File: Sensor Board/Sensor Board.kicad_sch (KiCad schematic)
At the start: 32 parts, among them J1 Programming Header, J3 Micro_SD_Card, U1 PIC18F26K83, U2 SPX3819M5-L-3-3, U3 MCP2562, Y1 12MHz Crystal

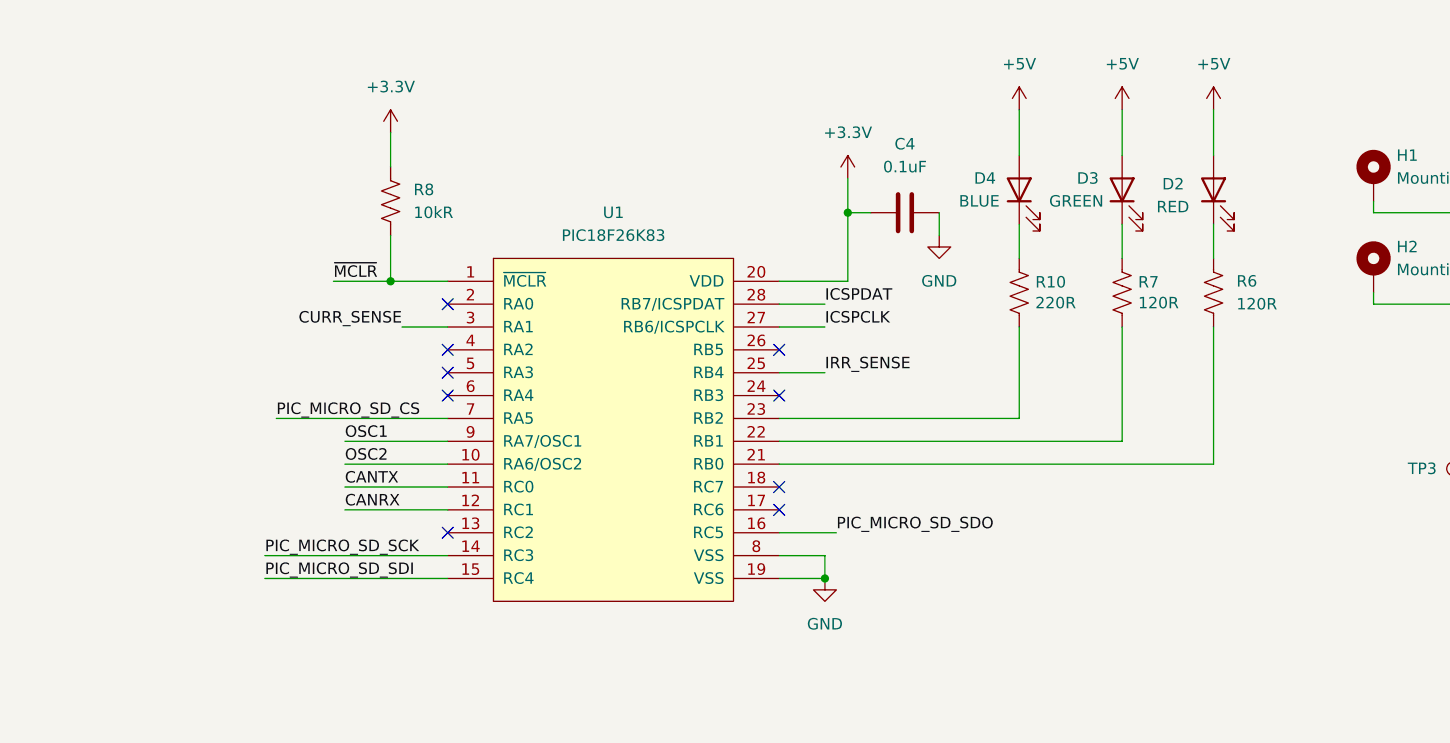
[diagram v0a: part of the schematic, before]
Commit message: Cooked another layout-Pranav
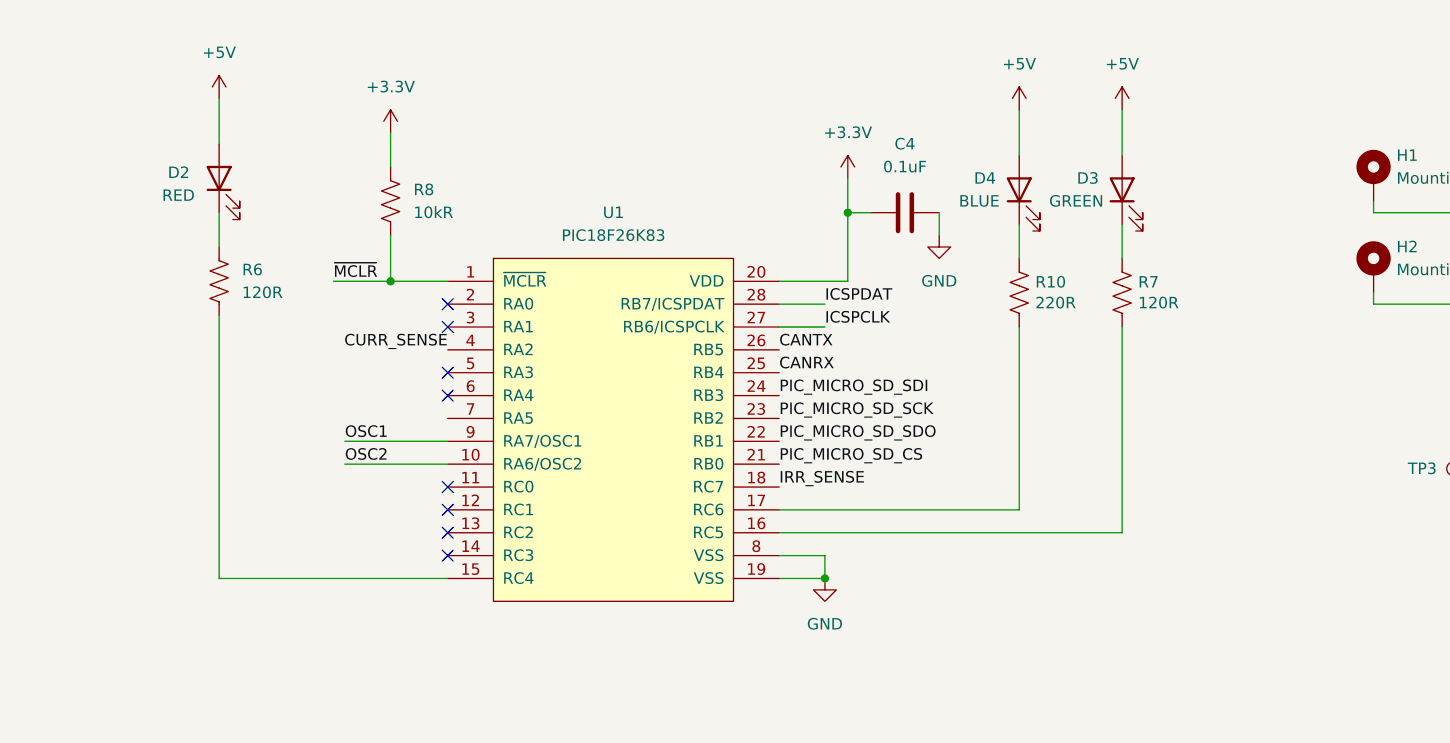
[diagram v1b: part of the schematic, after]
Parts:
- Y1: value 12MHz Crystal -> 12MHz Crystal
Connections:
- net CANRX: now also U1.25 (RB4); no longer U1.12 (RC1)
- net CANTX: now also U1.26 (RB5); no longer U1.11 (RC0)
- net CURR_SENSE: now also U1.4 (RA2); no longer U1.3 (RA1)
- net IRR_SENSE: now also U1.18 (RC7); no longer U1.25 (RB4)
- net PIC_MICRO_SD_CS: now also U1.21 (RB0); no longer U1.7 (RA5)
- net PIC_MICRO_SD_SCK: now also U1.23 (RB2); no longer U1.14 (RC3)
- net PIC_MICRO_SD_SDI: now also U1.24 (RB3); no longer U1.15 (RC4)
- net PIC_MICRO_SD_SDO: now also U1.22 (RB1); no longer U1.16 (RC5)
- net at U1.17 (RC6): now also R10.2
- net at R6.2: now also U1.15 (RC4); no longer U1.21 (RB0)
- net at R7.2: now also U1.16 (RC5); no longer U1.22 (RB1)
- no-connect marks 9 -> 8
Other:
- moved on the sheet: D2, R6
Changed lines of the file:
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@@
 	)
 	(no_connect
-		(at 162.56 73.66)
+		(at 125.73 78.74)
 	)
 	(no_connect
-		(at 125.73 60.96)
+		(at 125.73 53.34)
 	)
 	(no_connect
-		(at 162.56 71.12)
+		(at 125.73 60.96)
 	)
 	(no_connect
-		(at 125.73 50.8)
+		(at 125.73 73.66)
 	)
 	(no_connect
@@
 	)
 	(no_connect
-		(at 162.56 60.96)
-	)
-	(no_connect
-		(at 162.56 55.88)
+		(at 125.73 50.8)
 	)
 	(no_connect
@@
 	)
 	(no_connect
-		(at 125.73 55.88)
+		(at 125.73 71.12)
 	)
 	(wire
@@
 	(wire
 		(pts
-			(xy 200.66 29.21) (xy 200.66 34.29)
+			(xy 100.33 81.28) (xy 125.73 81.28)
 		)
 		(stroke
@@
 	(wire
 		(pts
-			(xy 120.65 53.34) (xy 125.73 53.34)
+			(xy 200.66 29.21) (xy 200.66 34.29)
 		)
 		(stroke
@@
 	(wire
 		(pts
-			(xy 210.82 29.21) (xy 210.82 34.29)
-		)
-		(stroke
-			(width 0)
-			(type default)
-		)
-	)
-	(wire
-		(pts
-			(xy 210.82 53.34) (xy 210.82 68.58)
+			(xy 100.33 27.94) (xy 100.33 33.02)
 		)
 		(stroke
@@
 	(wire
 		(pts
-			(xy 210.82 41.91) (xy 210.82 45.72)
+			(xy 100.33 40.64) (xy 100.33 44.45)
 		)
 		(stroke
@@
 	(wire
 		(pts
-			(xy 189.23 41.91) (xy 189.23 45.72)
+			(xy 200.66 53.34) (xy 200.66 76.2)
 		)
 		(stroke
@@
 	(wire
 		(pts
-			(xy 162.56 58.42) (xy 167.64 58.42)
+			(xy 189.23 41.91) (xy 189.23 45.72)
 		)
 		(stroke
@@
 	(wire
 		(pts
-			(xy 114.3 71.12) (xy 125.73 71.12)
-		)
-		(stroke
-			(width 0)
-			(type default)
-		)
-	)
-	(wire
-		(pts
 			(xy 85.09 134.62) (xy 85.09 138.43)
 		)
@@
 	(wire
 		(pts
-			(xy 162.56 66.04) (xy 200.66 66.04)
-		)
-		(stroke
-			(width 0)
-			(type default)
-		)
-	)
-	(wire
-		(pts
 			(xy 261.62 95.25) (xy 261.62 88.9)
 		)
@@
 	(wire
 		(pts
-			(xy 162.56 76.2) (xy 168.91 76.2)
-		)
-		(stroke
-			(width 0)
-			(type default)
-		)
-	)
-	(wire
-		(pts
 			(xy 125.73 115.57) (xy 125.73 113.03)
 		)
@@
 	(wire
 		(pts
-			(xy 105.41 81.28) (xy 125.73 81.28)
+			(xy 170.18 40.64) (xy 170.18 48.26)
 		)
 		(stroke
@@
 	(wire
 		(pts
-			(xy 170.18 40.64) (xy 170.18 48.26)
+			(xy 189.23 29.21) (xy 189.23 34.29)
 		)
 		(stroke
@@
 	(wire
 		(pts
-			(xy 189.23 29.21) (xy 189.23 34.29)
+			(xy 162.56 53.34) (xy 167.64 53.34)
 		)
 		(stroke
@@
 	(wire
 		(pts
-			(xy 162.56 53.34) (xy 167.64 53.34)
+			(xy 248.92 115.57) (xy 251.46 115.57)
 		)
 		(stroke
@@
 	(wire
 		(pts
-			(xy 248.92 115.57) (xy 251.46 115.57)
+			(xy 237.49 72.39) (xy 237.49 77.47)
 		)
 		(stroke
@@
 	(wire
 		(pts
-			(xy 237.49 72.39) (xy 237.49 77.47)
+			(xy 100.33 52.07) (xy 100.33 81.28)
 		)
 		(stroke
@@
 	(wire
 		(pts
-			(xy 200.66 53.34) (xy 200.66 66.04)
+			(xy 162.56 73.66) (xy 189.23 73.66)
 		)
 		(stroke
@@
 	(wire
 		(pts
-			(xy 189.23 53.34) (xy 189.23 63.5)
+			(xy 189.23 53.34) (xy 189.23 73.66)
 		)
 		(stroke
@@
 	(wire
 		(pts
-			(xy 114.3 73.66) (xy 125.73 73.66)
-		)
-		(stroke
-			(width 0)
-			(type default)
-		)
-	)
-	(wire
-		(pts
 			(xy 200.66 45.72) (xy 200.66 41.91)
 		)
@@
 	(wire
 		(pts
-			(xy 105.41 78.74) (xy 125.73 78.74)
-		)
-		(stroke
-			(width 0)
-			(type default)
-		)
-	)
-	(wire
-		(pts
 			(xy 144.78 113.03) (xy 166.37 113.03)
 		)
@@
 	(wire
 		(pts
-			(xy 21.59 119.38) (xy 21.59 123.19)
+			(xy 200.66 76.2) (xy 162.56 76.2)
 		)
 		(stroke
@@
 	(wire
 		(pts
-			(xy 172.72 40.64) (xy 170.18 40.64)
+			(xy 21.59 119.38) (xy 21.59 123.19)
 		)
 		(stroke
@@
 	(wire
 		(pts
-			(xy 106.68 63.5) (xy 125.73 63.5)
+			(xy 172.72 40.64) (xy 170.18 40.64)
 		)
 		(stroke
@@
 	(wire
 		(pts
-			(xy 162.56 68.58) (xy 210.82 68.58)
-		)
-		(stroke
-			(width 0)
-			(type default)
-		)
-	)
-	(wire
-		(pts
 			(xy 114.3 66.04) (xy 125.73 66.04)
 		)
@@
 	(wire
 		(pts
-			(xy 189.23 63.5) (xy 162.56 63.5)
-		)
-		(stroke
-			(width 0)
-			(type default)
-		)
-	)
-	(wire
-		(pts
 			(xy 48.26 181.61) (xy 48.26 161.29)
 		)
@@
 	)
 	(label "IRR_SENSE"
-		(at 167.64 58.42 0)
+		(at 162.56 71.12 0)
 		(fields_autoplaced yes)
 		(effects
@@
 	)
 	(label "CANTX"
-		(at 114.3 71.12 0)
+		(at 162.56 55.88 0)
 		(fields_autoplaced yes)
 		(effects
@@
 	)
 	(label "PIC_MICRO_SD_SCK"
-		(at 105.41 78.74 0)
+		(at 162.56 63.5 0)
 		(fields_autoplaced yes)
 		(effects
@@
 	)
 	(label "CANRX"
-		(at 114.3 73.66 0)
+		(at 162.56 58.42 0)
 		(fields_autoplaced yes)
 		(effects
@@
 	)
 	(label "PIC_MICRO_SD_SDO"
-		(at 168.91 76.2 0)
+		(at 162.56 66.04 0)
 		(fields_autoplaced yes)
 		(effects
@@
 	)
 	(label "PIC_MICRO_SD_SDI"
-		(at 105.41 81.28 0)
+		(at 162.56 60.96 0)
 		(fields_autoplaced yes)
 		(effects
@@
 	)
 	(label "PIC_MICRO_SD_CS"
-		(at 106.68 63.5 0)
+		(at 162.56 68.58 0)
 		(fields_autoplaced yes)
 		(effects
@@
 	)
 	(label "CURR_SENSE"
-		(at 120.65 53.34 180)
+		(at 125.73 55.88 180)
 		(fields_autoplaced yes)
 		(effects
@@
 			)
 		)
-		(property "Value" "12MHz Crystal "
+		(property "Value" "12MHz Crystal"
 			(at 38.8874 111.633 90)
 			(effects
@@
 		(lib_name "+5V_3")
 		(lib_id "power:+5V")
-		(at 210.82 29.21 0)
+		(at 100.33 27.94 0)
 		(unit 1)
 		(exclude_from_sim no)
@@
 		(fields_autoplaced yes)
 		(property "Reference" "#PWR06"
-			(at 210.82 33.02 0)
+			(at 100.33 31.75 0)
 			(effects
 				(font
@@
 		)
 		(property "Value" "+5V"
-			(at 210.82 24.13 0)
+			(at 100.33 22.86 0)
 			(effects
 				(font
@@
 		)
 		(property "Footprint" ""
-			(at 210.82 29.21 0)
+			(at 100.33 27.94 0)
 			(effects
 				(font
@@
 		)
 		(property "Datasheet" ""
-			(at 210.82 29.21 0)
+			(at 100.33 27.94 0)
 			(effects
 				(font
@@
 		)
 		(property "Description" "Power symbol creates a global label with name \"+5V\""
-			(at 210.82 29.21 0)
+			(at 100.33 27.94 0)
 			(effects
 				(font
@@
 	(symbol
 		(lib_id "Device:LED")
-		(at 210.82 38.1 90)
+		(at 100.33 36.83 90)
 		(unit 1)
 		(exclude_from_sim no)
@@
 		(dnp no)
 		(property "Reference" "D2"
-			(at 205.105 37.465 90)
+			(at 94.615 36.195 90)
 			(effects
 				(font
@@
 		)
 		(property "Value" "RED"
-			(at 204.47 40.005 90)
+			(at 93.98 38.735 90)
 			(effects
 				(font
@@
 		)
 		(property "Footprint" "LED_SMD:LED_1206_3216Metric_Pad1.42x1.75mm_HandSolder"
-			(at 210.82 38.1 0)
+			(at 100.33 36.83 0)
 			(effects
 				(font
@@
 		)
 		(property "Datasheet" "~"
-			(at 210.82 38.1 0)
+			(at 100.33 36.83 0)
 			(effects
 				(font
@@
 		)
 		(property "Description" ""
-			(at 210.82 38.1 0)
+			(at 100.33 36.83 0)
 			(effects
 				(font
@@
 		)
 		(property "DigiKey" "160-1457-1-ND"
-			(at 210.82 38.1 90)
+			(at 100.33 36.83 90)
 			(effects
 				(font
@@
 	(symbol
 		(lib_id "Device:R_US")
-		(at 210.82 49.53 0)
+		(at 100.33 48.26 0)
 		(unit 1)
 		(exclude_from_sim no)
@@
 		(fields_autoplaced yes)
 		(property "Reference" "R6"
-			(at 213.36 48.2599 0)
+			(at 102.87 46.9899 0)
 			(effects
 				(font
@@
 		)
 		(property "Value" "120R"
-			(at 213.36 50.7999 0)
+			(at 102.87 49.5299 0)
 			(effects
 				(font
@@
 		)
 		(property "Footprint" "Resistor_SMD:R_0805_2012Metric_Pad1.20x1.40mm_HandSolder"
-			(at 211.836 49.784 90)
+			(at 101.346 48.514 90)
 			(effects
 				(font
@@
 		)
 		(property "Datasheet" "~"
-			(at 210.82 49.53 0)
+			(at 100.33 48.26 0)
 			(effects
 				(font
@@
 		)
 		(property "Description" ""
-			(at 210.82 49.53 0)
+			(at 100.33 48.26 0)
 			(effects
 				(font
@@
 		)
 		(property "DigiKey" "738-RMCF0805FT160RCT-ND"
-			(at 210.82 49.53 0)
+			(at 100.33 48.26 0)
 			(effects
 				(font

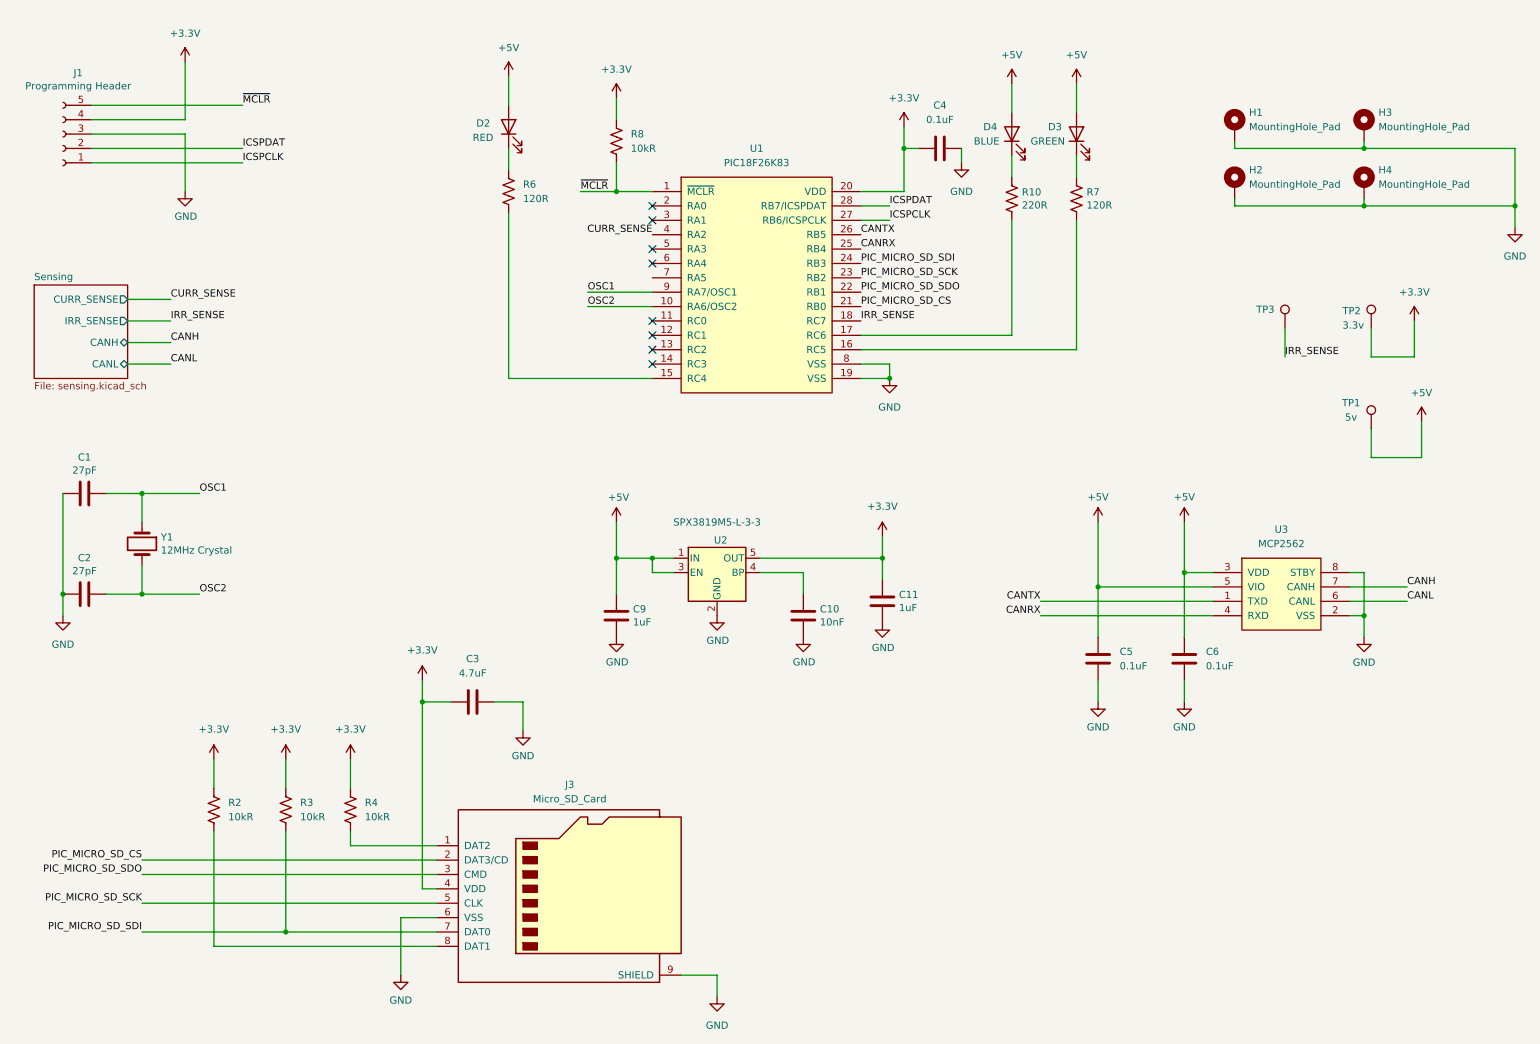
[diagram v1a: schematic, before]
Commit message: updated optics front end
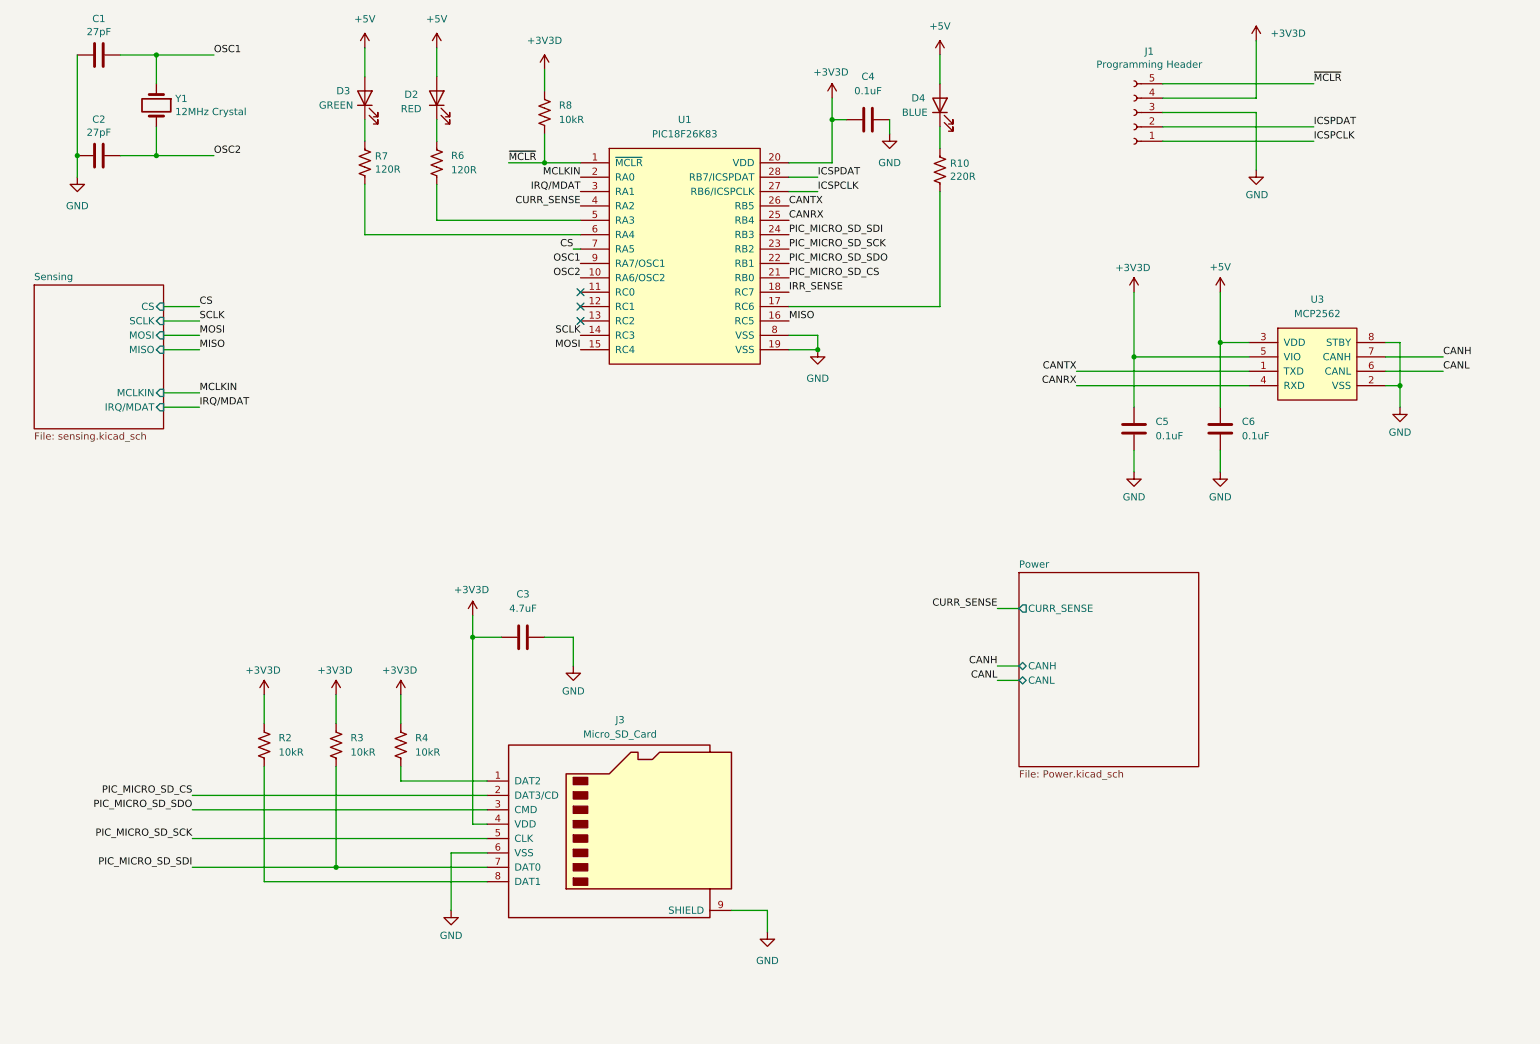
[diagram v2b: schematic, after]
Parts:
- removed C10: 10nF, Capacitor_SMD:C_0805_2012Metric_Pad1.18x1.45mm_HandSolder, symbol Device:C
- removed C11, C9: 1uF, Capacitor_SMD:C_0805_2012Metric_Pad1.18x1.45mm_HandSolder, symbol Device:C
- removed H1, H2, H3, H4: MountingHole_Pad, MountingHole:MountingHole_3.2mm_M3_DIN965_Pad, symbol Mechanical:MountingHole_Pad
- removed TP1: 5v, TestPoint:TestPoint_Pad_1.5x1.5mm, symbol Connector:TestPoint
- removed TP2: 3.3v, TestPoint:TestPoint_Pad_1.5x1.5mm, symbol Connector:TestPoint
- removed TP3: TestPoint, TestPoint:TestPoint_Pad_1.5x1.5mm, symbol Connector:TestPoint
- removed U2: SPX3819M5-L-3-3, Package_TO_SOT_SMD:SOT-23-5_HandSoldering, symbol Regulator_Linear:SPX3819M5-L-3-3
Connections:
- net +5V: no longer C5.2, U3.5 (VIO)
- net SCLK: now reaches U1.14 (RC3)
- net at R6.2: now also U1.5 (RA3); no longer U1.15 (RC4)
- net at R7.2: now also U1.6 (RA4); no longer U1.16 (RC5)
- net MCLKIN: now reaches U1.2 (RA0)
- net IRQ/MDAT: now reaches U1.3 (RA1)
- net CS: now reaches U1.7 (RA5)
- net +3.3V renamed +3V3D
- net +3V3D: now also C5.2, U3.5 (VIO)
- new net MISO: U1.16 (RC5)
- new net MOSI: U1.15 (RC4)
- no-connect marks 8 -> 3
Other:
- added sheet Power (Power.kicad_sch)
- sheet Sensing ports: added CS, IRQ/MDAT, MCLKIN, MISO, MOSI, SCLK; removed CANH, CANL, CURR_SENSE, IRR_SENSE
- moved on the sheet: C1, C2, C3, C4, C5, C6, D2, D3, D4, J1, J3, R10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
